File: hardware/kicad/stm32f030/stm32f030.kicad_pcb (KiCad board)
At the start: 2 copper layers, 67.3 x 68.6 mm, 114 parts, among them IC1 AT24CS02-SSHM, K1 RELAY_1RT, K2 RELAY_1RT, P1 5VIN, P10 SWD, P2 LOOP1, P3 LOOP2, P4 RELAY OUT 1, P5 TTL OUT 1, P6 RELAY OUT 2, P7 TTL OUT 2, P8 UART, P9 I2C, Q1 BSS138, Q2 BC817-40, Q3 BSS138, Q4 BC817-40, Q5 BC817-40, Q6 BC817-40, Q7 BC817-40, Q8 BC817-40, SW1 TACTILE_SW, SW2 TACTILE_SW, SW3 RESET, T1 78601/9C, T2 78601/9C, U1 LM1117-3.3, U2 STM32F030F4Px, U3 MCP23017, Y1 12MHz

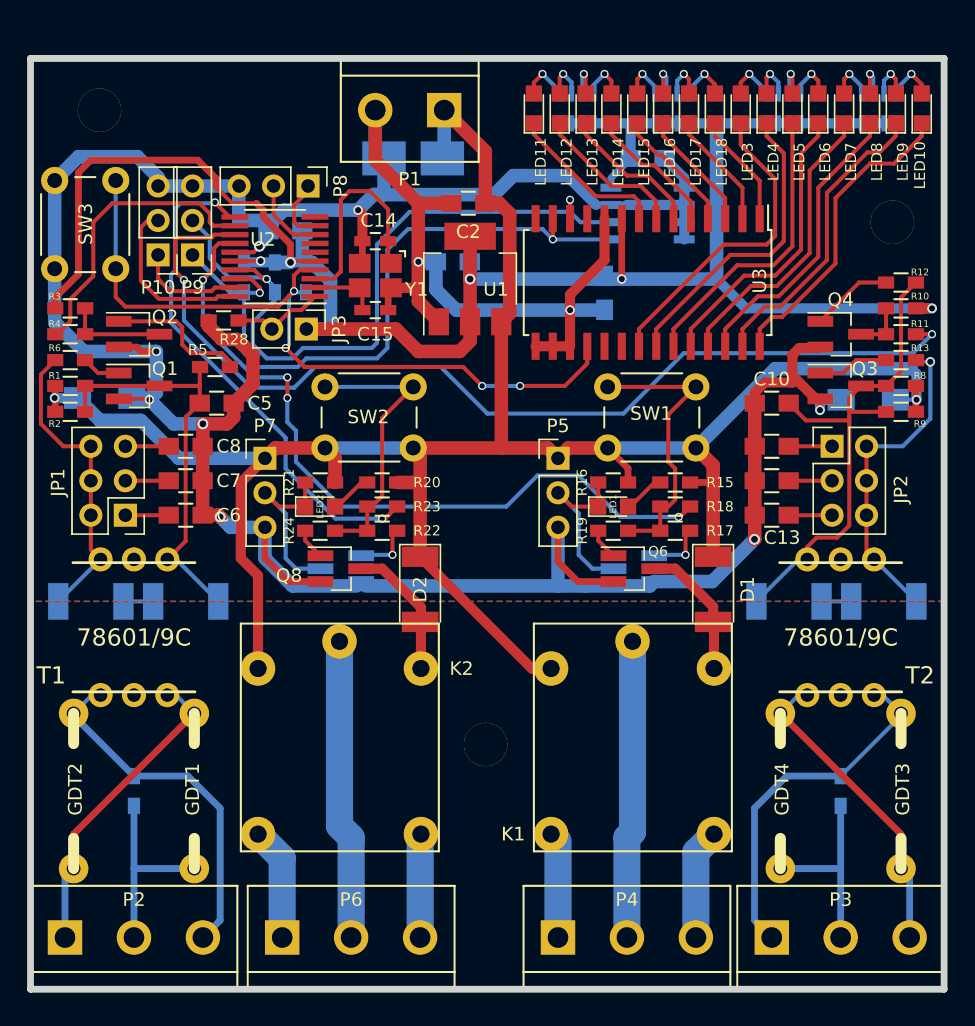
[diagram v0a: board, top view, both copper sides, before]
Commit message: hardware/kicad/stm32f030: final touches
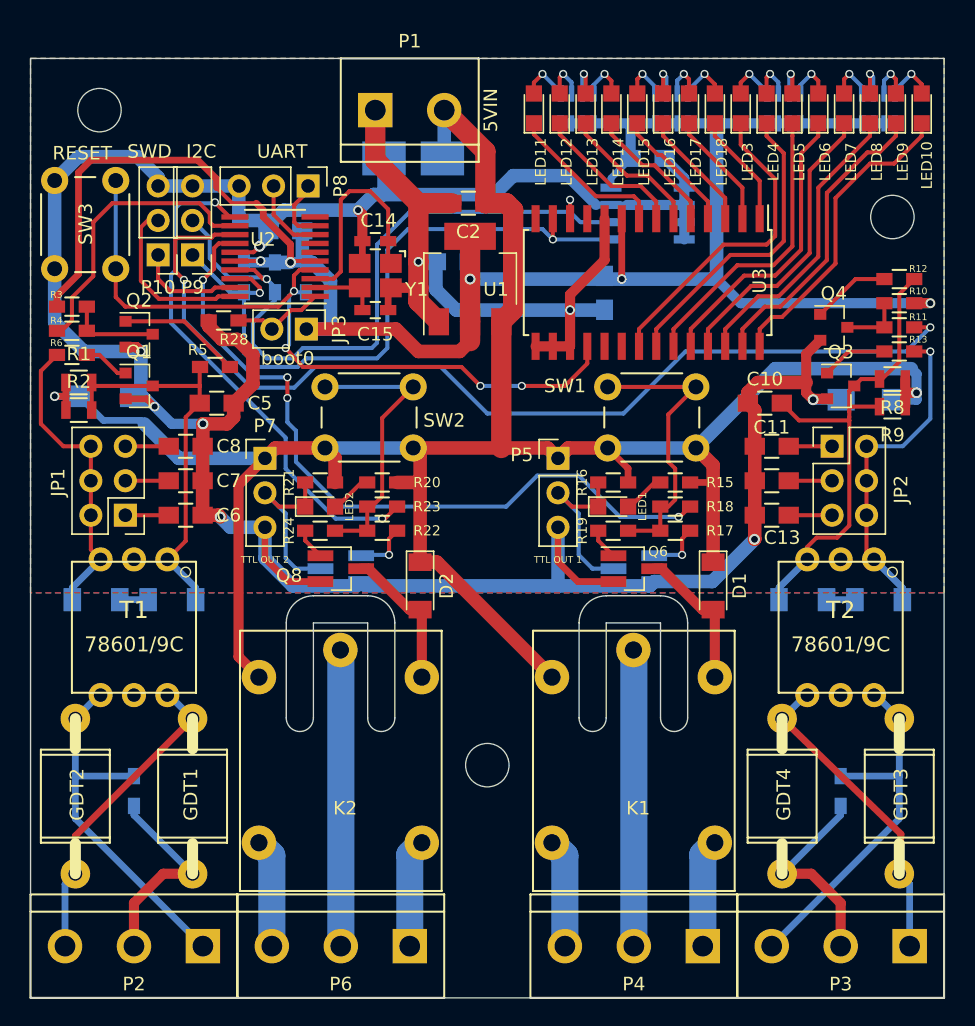
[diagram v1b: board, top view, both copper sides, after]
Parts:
- D1, D2, ZD1, ZD2, ZD3, ZD4: footprint Diodes_SMD:MELF_Standard -> Diodes_SMD:D_MiniMELF_Standard
- Q1, Q2, Q3, Q4: footprint TO_SOT_Packages_SMD:SOT-23_Handsoldering -> TO_SOT_Packages_SMD:SOT-23
- R1, R2, R8, R9: footprint Resistors_SMD:R_0603_HandSoldering -> Resistors_SMD:R_0805
- T1, T2: footprint cardetector:78601_9C -> cardetector:Murata_Impulse_Transformer
- moved REF** 1.53 mm to (69.2, 144.8)
- moved ZD1 1.02 mm to (46.0, 132.6)
- moved ZD3 1.02 mm to (92.5, 132.6)
- moved P6 0.99 mm to (58.4, 158.1), turned to 180 degrees
- moved P4 0.81 mm to (80.0, 158.1), turned to 180 degrees
- moved R8 0.81 mm to (99.1, 116.3)
- moved R9 0.74 mm to (99.1, 118.4)
- moved Q4 0.72 mm to (94.7, 112.5)
- moved R1 0.68 mm to (39.1, 116.6)
- moved R13 0.65 mm to (99.6, 114.3)
- moved R2 0.65 mm to (39.1, 118.6)
- moved K1 0.64 mm to (74.0, 150.5)
- moved K2 0.64 mm to (52.4, 150.5)
- moved P2 0.64 mm to (43.2, 158.1), turned to 180 degrees
- moved P3 0.64 mm to (95.2, 158.1), turned to 180 degrees
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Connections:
- P1 pad 1: +5V -> GND
- P1 pad 2: GND -> +5V
- P2 pad 1: Net-(GDT1-Pad1) -> Net-(GDT2-Pad1)
- P2 pad 3: Net-(GDT2-Pad1) -> Net-(GDT1-Pad1)
- P3 pad 1: Net-(GDT3-Pad1) -> Net-(GDT3-Pad2)
- P3 pad 3: Net-(GDT3-Pad2) -> Net-(GDT3-Pad1)
- P4 pad 1: Net-(K1-Pad3) -> Net-(K1-Pad4)
- P4 pad 3: Net-(K1-Pad4) -> Net-(K1-Pad3)
- P6 pad 1: Net-(K2-Pad3) -> Net-(K2-Pad4)
- P6 pad 3: Net-(K2-Pad4) -> Net-(K2-Pad3)
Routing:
- net +5V: track 163.8 -> 169.3 mm
- net GND: track 269.2 -> 266.0 mm
- net Net-(C5-Pad1): track 30.6 -> 29.1 mm
- net Net-(Q2-Pad1): track 10.6 -> 9.08 mm
- net Net-(GDT3-Pad1): track 26.4 -> 27.7 mm
- net Net-(GDT2-Pad1): track 26.4 -> 27.6 mm
- net Net-(C10-Pad1): track 38.4 -> 37.3 mm
- net Net-(GDT4-Pad2): track 14.1 -> 15.2 mm
- net Net-(GDT1-Pad2): track 14.1 -> 15.2 mm
- net Net-(JP1-Pad2): track 23.5 -> 22.5 mm
- net Net-(Q4-Pad3): track 3.75 -> 4.50 mm
- net Net-(Q2-Pad3): track 7.38 -> 6.74 mm
- net Net-(Q1-Pad1): track 2.88 -> 3.41 mm
- net Net-(D2-Pad2): track 10.1 -> 10.6 mm
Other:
- board size 67.3 x 68.6 mm -> 67.3 x 69.2 mm
